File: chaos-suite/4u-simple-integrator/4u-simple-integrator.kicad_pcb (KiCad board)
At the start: 2 copper layers, 50.8 x 149.9 mm, 39 parts, among them J1 BananaJack_PanelMount, J10 I2_Main, J11 4U_Power, J2 BananaJack_PanelMount, J3 BananaJack_PanelMount, J4 BananaJack_PanelMount, J5 BananaJack_PanelMount, J6 BananaJack_PanelMount, J7 I1_Ctrl, J8 I2_Ctrl, J9 I1_Main, U1 TL074

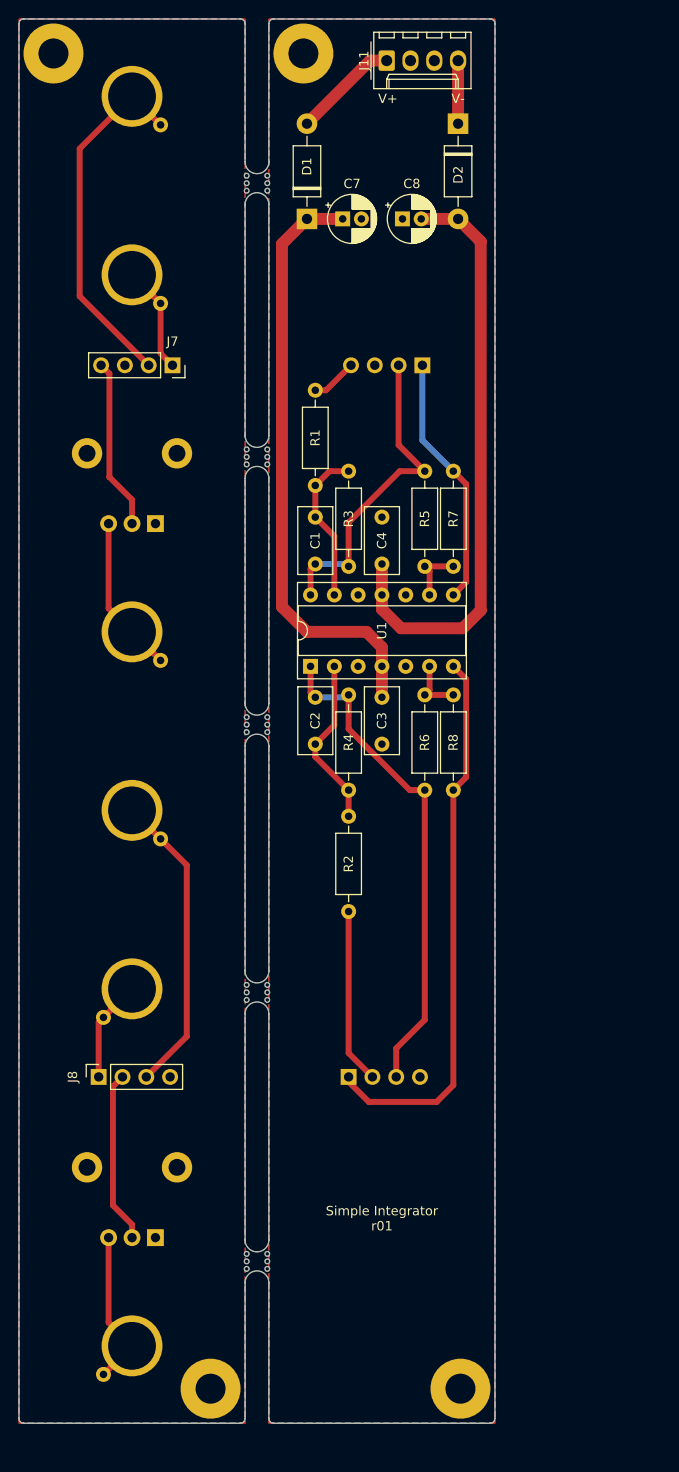
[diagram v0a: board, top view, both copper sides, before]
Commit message: Updating simple integrator to rev2
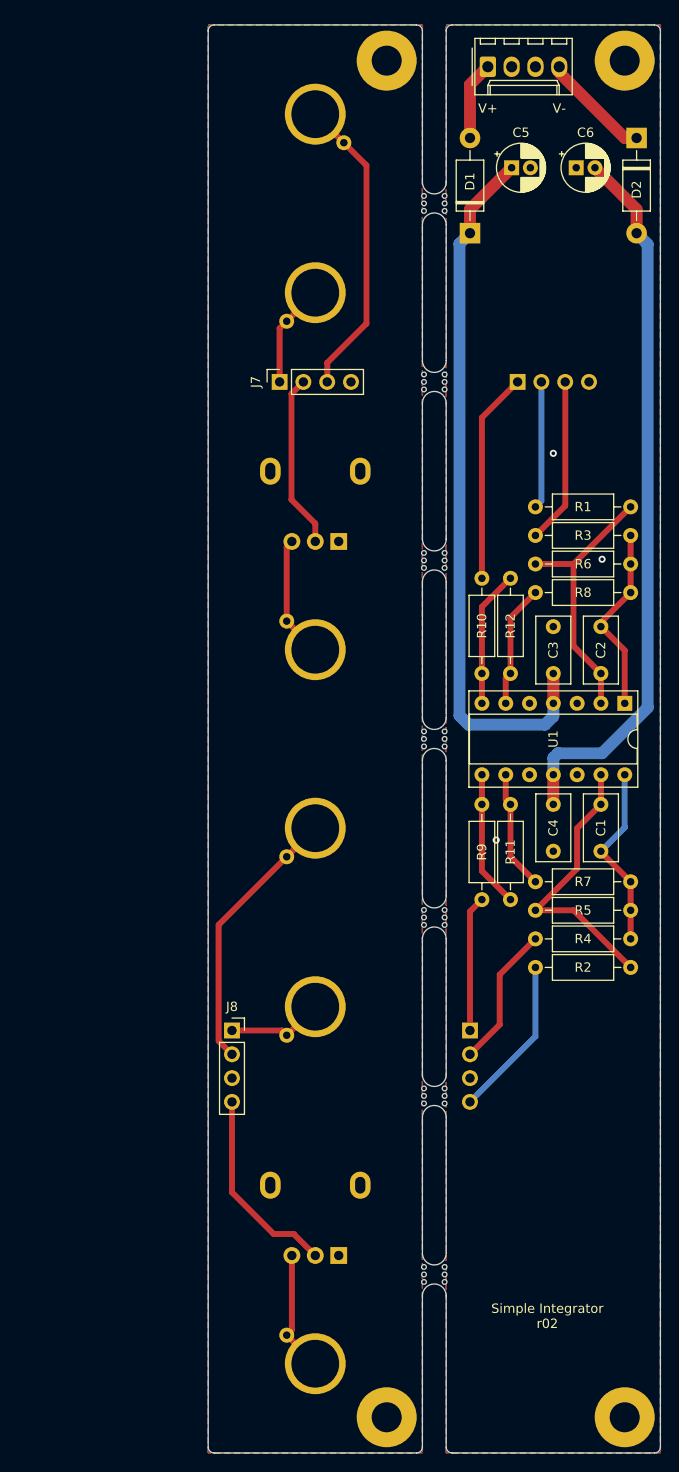
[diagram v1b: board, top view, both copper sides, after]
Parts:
- removed C7, C8: 1uF, Capacitor_THT:CP_Radial_D5.0mm_P2.00mm
- removed H5, H6, H7, H8, H9: MouseBite, Panelization:mouse-bite-2.54mm-slot
- added C5: 10uF, rumblesan-standard-parts:CP_Radial_D5.0mm_P2.00mm, F.Cu at (126.4, 47.0)
- added C6: 10uF, rumblesan-standard-parts:CP_Radial_D5.0mm_P2.00mm, F.Cu at (133.3, 47.0)
- added R10: 330r, rumblesan-standard-parts:R_Axial_DIN0207_L6.3mm_D2.5mm_P10.16mm_Horizontal, F.Cu at (123.2, 90.8)
- added R11: 10k, rumblesan-standard-parts:R_Axial_DIN0207_L6.3mm_D2.5mm_P10.16mm_Horizontal, F.Cu at (126.2, 125.1)
- added R12: 10k, rumblesan-standard-parts:R_Axial_DIN0207_L6.3mm_D2.5mm_P10.16mm_Horizontal, F.Cu at (126.2, 90.8)
- added R9: 330r, rumblesan-standard-parts:R_Axial_DIN0207_L6.3mm_D2.5mm_P10.16mm_Horizontal, F.Cu at (123.2, 125.1)
- added mouse-bite-2.54mm-slot: VAL**, Panelization:mouse-bite-2.54mm-slot, F.Cu at (118.1, 165.1)
- added mouse-bite-2.54mm-slot: VAL**, Panelization:mouse-bite-2.54mm-slot, F.Cu at (118.1, 146.1)
- added mouse-bite-2.54mm-slot: VAL**, Panelization:mouse-bite-2.54mm-slot, F.Cu at (118.1, 50.8)
- added mouse-bite-2.54mm-slot: VAL**, Panelization:mouse-bite-2.54mm-slot, F.Cu at (118.1, 127.0)
- added mouse-bite-2.54mm-slot: VAL**, Panelization:mouse-bite-2.54mm-slot, F.Cu at (118.1, 69.8)
- added mouse-bite-2.54mm-slot: VAL**, Panelization:mouse-bite-2.54mm-slot, F.Cu at (118.1, 108.0)
- added mouse-bite-2.54mm-slot: VAL**, Panelization:mouse-bite-2.54mm-slot, F.Cu at (118.1, 88.9)
- C1, C2: value 1nF (poly) -> 1nF; footprint Rumblesan_Footprints:C_Rect_L7.0mm_W3.5mm_P5.00mm -> rumblesan-standard-parts:C_Rect_L7.0mm_W3.5mm_P5.00mm
- C3, C4: value 100nF (X7R) -> 100nF; footprint Rumblesan_Footprints:C_Rect_L7.0mm_W3.5mm_P5.00mm -> rumblesan-standard-parts:C_Rect_L7.0mm_W3.5mm_P5.00mm
- D1, D2: footprint Rumblesan_Footprints:D_DO-41_SOD81_P10.16mm_Horizontal -> rumblesan-standard-parts:D_DO-41_SOD81_P10.16mm_Horizontal
- J1, J2, J3, J4, J5, J6: footprint Rumblesan_Footprints:BananaJack_THT_JohnsonCinch_108-09 -> rumblesan-standard-parts:BananaJack_THT_JohnsonCinch_108-09
- J10: value I2_Main -> I1_Main
- J11: footprint Rumblesan_Footprints:4u_Power_Molex_KK-254_P2.54mm -> 4u-power:4u_Power_Molex_KK-254_P2.54mm
- J7: value I1_Ctrl -> I2_Ctrl
- J8: value I2_Ctrl -> I1_Ctrl
- J9: value I1_Main -> I2_Main
- R1, R2, R7, R8: footprint Rumblesan_Footprints:Resistor_THT_L6.3mm_D2.5mm_P10.16mm_Horizontal -> rumblesan-standard-parts:R_Axial_DIN0207_L6.3mm_D2.5mm_P10.16mm_Horizontal
- R3, R4: value 100k -> 330r; footprint Rumblesan_Footprints:Resistor_THT_L6.3mm_D2.5mm_P10.16mm_Horizontal -> rumblesan-standard-parts:R_Axial_DIN0207_L6.3mm_D2.5mm_P10.16mm_Horizontal
- R5, R6: value 10k -> 100k (optional); footprint Rumblesan_Footprints:Resistor_THT_L6.3mm_D2.5mm_P10.16mm_Horizontal -> rumblesan-standard-parts:R_Axial_DIN0207_L6.3mm_D2.5mm_P10.16mm_Horizontal
- RV1, RV2: footprint Rumblesan_Footprints:Potentiometer_Alpha_RD901F-40-00D_Single_Vertical_CircularHoles -> rumblesan-standard-parts:Potentiometer_Alpha_RD901F-40-00D_Single_Vertical
- U1: footprint Rumblesan_Footprints:DIP-14_W7.62mm_Socket -> rumblesan-standard-parts:DIP-14_W7.62mm_Socket
- moved R5 51.8 mm to (139.1, 126.2), turned to 180 degrees
- moved C1 43.2 mm to (135.9, 114.9)
- moved C4 40.1 mm to (130.8, 119.9), turned to 90 degrees
- moved R1 35.9 mm to (139.1, 83.2), turned to 180 degrees
- moved H4 35.6 mm to (113.0, 35.6)
- moved R7 34.8 mm to (128.9, 123.2), turned to 0 degrees
- moved H2 34.3 mm to (138.4, 35.6)
- moved U1 33.8 mm to (138.4, 104.2), turned to -90 degrees
- moved R6 32.6 mm to (139.1, 89.3), turned to 180 degrees
- moved C2 31.4 mm to (135.9, 101.0)
- moved R2 30.7 mm to (139.1, 132.3), turned to 180 degrees
- moved R4 25.5 mm to (128.9, 129.3), turned to 0 degrees
- moved R3 21.1 mm to (128.9, 86.2), turned to 0 degrees
- moved J1 19.7 mm to (105.4, 98.4), turned to 180 degrees
- moved J2 19.7 mm to (105.4, 174.6), turned to 180 degrees
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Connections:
- C2 pad 1: Net-(R2-Pad2) -> Net-(C2-Pad1)
- J10 pad 3: Net-(C2-Pad2) -> GND
- J10 pad 4: GND -> Net-(J10-Pad4)
- J7 pad 2: Net-(J4-Pad1) -> Net-(J7-Pad2)
- J7 pad 3: GND -> Net-(J4-Pad1)
- J7 pad 4: Net-(RV1-Pad2) -> GND
- J8 pad 2: Net-(J8-Pad2) -> Net-(J6-Pad1)
- J8 pad 3: Net-(J6-Pad1) -> GND
- J8 pad 4: GND -> Net-(J8-Pad4)
- J9 pad 1: Net-(R7-Pad2) -> Net-(J9-Pad1)
- J9 pad 2: Net-(C1-Pad2) -> Net-(J9-Pad2)
- J9 pad 3: GND -> Net-(J9-Pad3)
- J9 pad 4: Net-(R1-Pad1) -> GND
- R1 pad 1: Net-(R1-Pad1) -> Net-(C2-Pad1)
- R1 pad 2: Net-(C1-Pad1) -> Net-(J9-Pad2)
- R2 pad 1: Net-(J10-Pad2) -> Net-(C1-Pad1)
- R2 pad 2: Net-(R2-Pad2) -> Net-(J10-Pad4)
- R3 pad 1: Net-(C1-Pad1) -> Net-(J9-Pad3)
- R3 pad 2: Net-(C1-Pad2) -> Net-(C2-Pad2)
- R4 pad 1: Net-(R2-Pad2) -> Net-(J10-Pad2)
- R4 pad 2: Net-(C2-Pad2) -> Net-(C1-Pad2)
- R5 pad 2: Net-(R5-Pad2) -> Net-(C1-Pad1)
- R6 pad 2: Net-(R6-Pad2) -> Net-(C2-Pad1)
- R7 pad 1: Net-(R5-Pad2) -> Net-(R11-Pad2)
- R7 pad 2: Net-(R7-Pad2) -> Net-(C1-Pad2)
- R8 pad 1: Net-(R6-Pad2) -> Net-(R12-Pad2)
- R8 pad 2: Net-(J10-Pad1) -> Net-(C2-Pad2)
- RV1 pad 2: Net-(RV1-Pad2) -> Net-(J7-Pad2)
- RV2 pad 2: Net-(J8-Pad2) -> Net-(J8-Pad4)
- U1 pad 2: Net-(R2-Pad2) -> Net-(C2-Pad1)
- U1 pad 6: Net-(R6-Pad2) -> Net-(R12-Pad2)
- U1 pad 7: Net-(J10-Pad1) -> Net-(R10-Pad2)
- U1 pad 8: Net-(R7-Pad2) -> Net-(R11-Pad1)
- U1 pad 9: Net-(R5-Pad2) -> Net-(R11-Pad2)
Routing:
- net Net-(J10-Pad1): track 59.2 -> 14.5 mm
- net Net-(C2-Pad2): track 53.5 -> 20.3 mm
- net Net-(C2-Pad1): track 0.00 -> 28.8 mm
- net Net-(R7-Pad2): track 27.0 -> 0.00 mm
- net Net-(J9-Pad1): track 0.00 -> 22.5 mm
- net Net-(J8-Pad4): track 0.00 -> 21.3 mm
- net Net-(J7-Pad2): track 0.00 -> 18.6 mm
- net Net-(J8-Pad2): track 18.4 -> 0.00 mm
- net Net-(R2-Pad2): track 18.3 -> 0.00 mm
- net Net-(RV1-Pad2): track 18.3 -> 0.00 mm
- net Net-(J9-Pad3): track 0.00 -> 17.7 mm
- net Net-(J10-Pad4): track 0.00 -> 17.2 mm
- net Net-(C1-Pad2): track 34.7 -> 19.9 mm
- net Net-(R10-Pad2): track 0.00 -> 14.6 mm
- net Net-(R11-Pad1): track 0.00 -> 14.6 mm
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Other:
- board size 50.8 x 149.9 mm -> 48.3 x 152.4 mm
- board text added: "Simple Integrator r02"
- board text removed: "Simple Integrator r01"
